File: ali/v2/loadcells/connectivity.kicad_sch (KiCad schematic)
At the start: 27 parts, among them J7 Conn_01x03, J8 Vertical Ethernet, U3 TJA1462ATK, U4 LAN8742AI, Y3 25 MHz

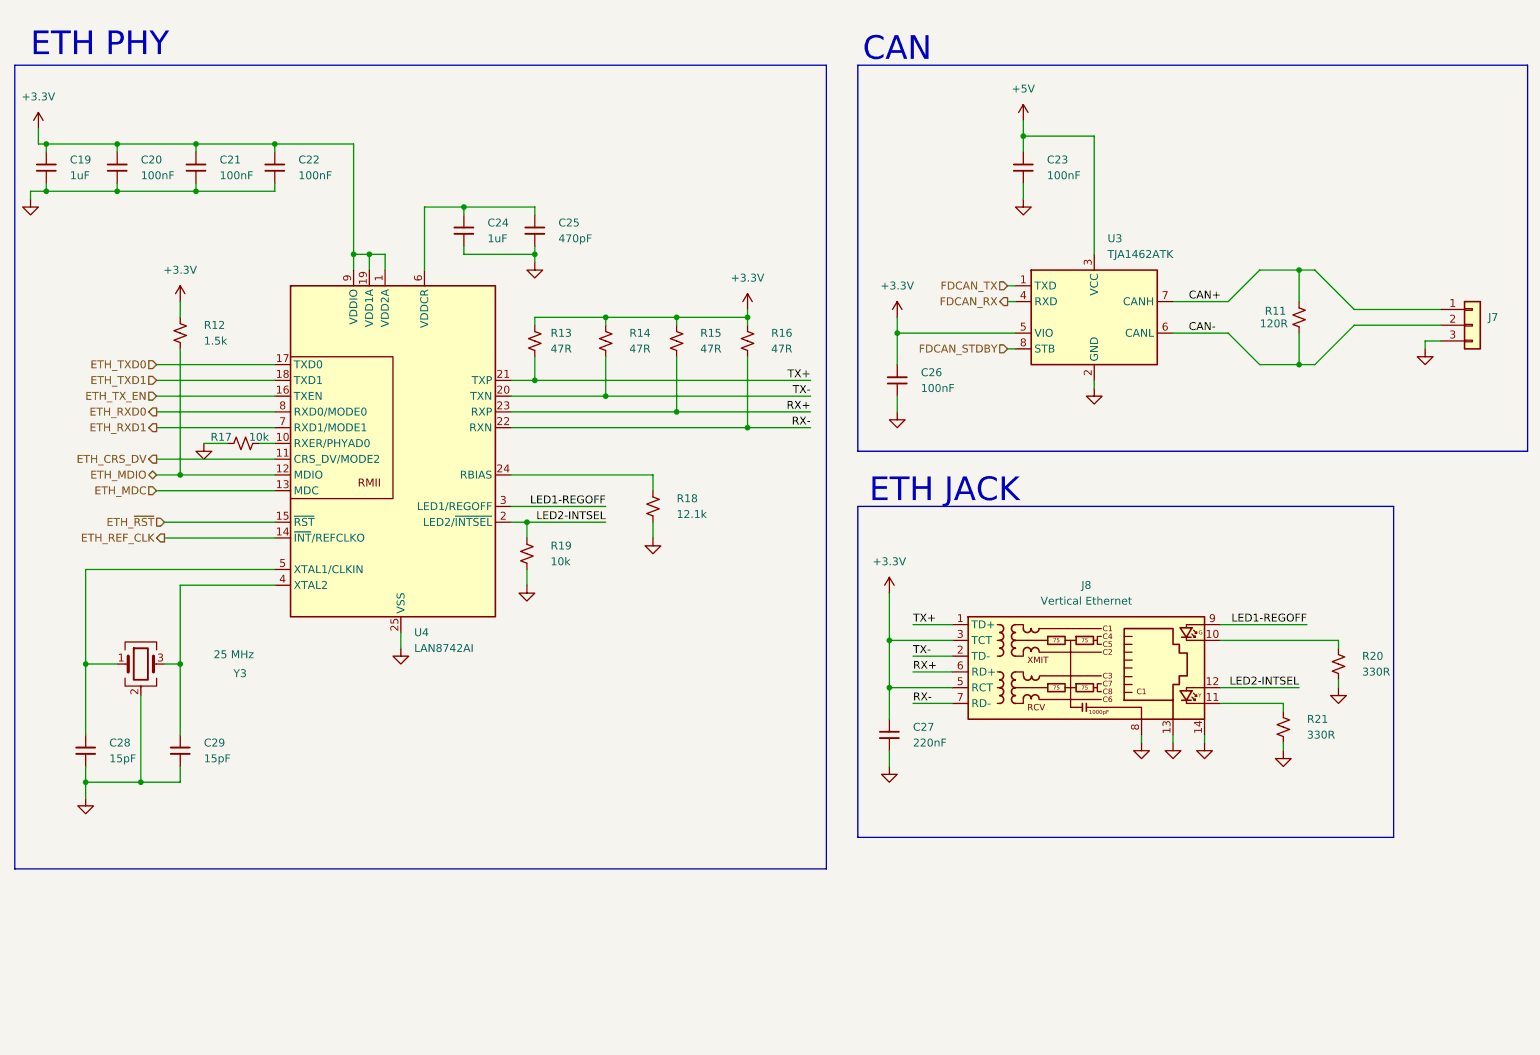
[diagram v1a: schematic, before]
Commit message: Begin prep for second board review
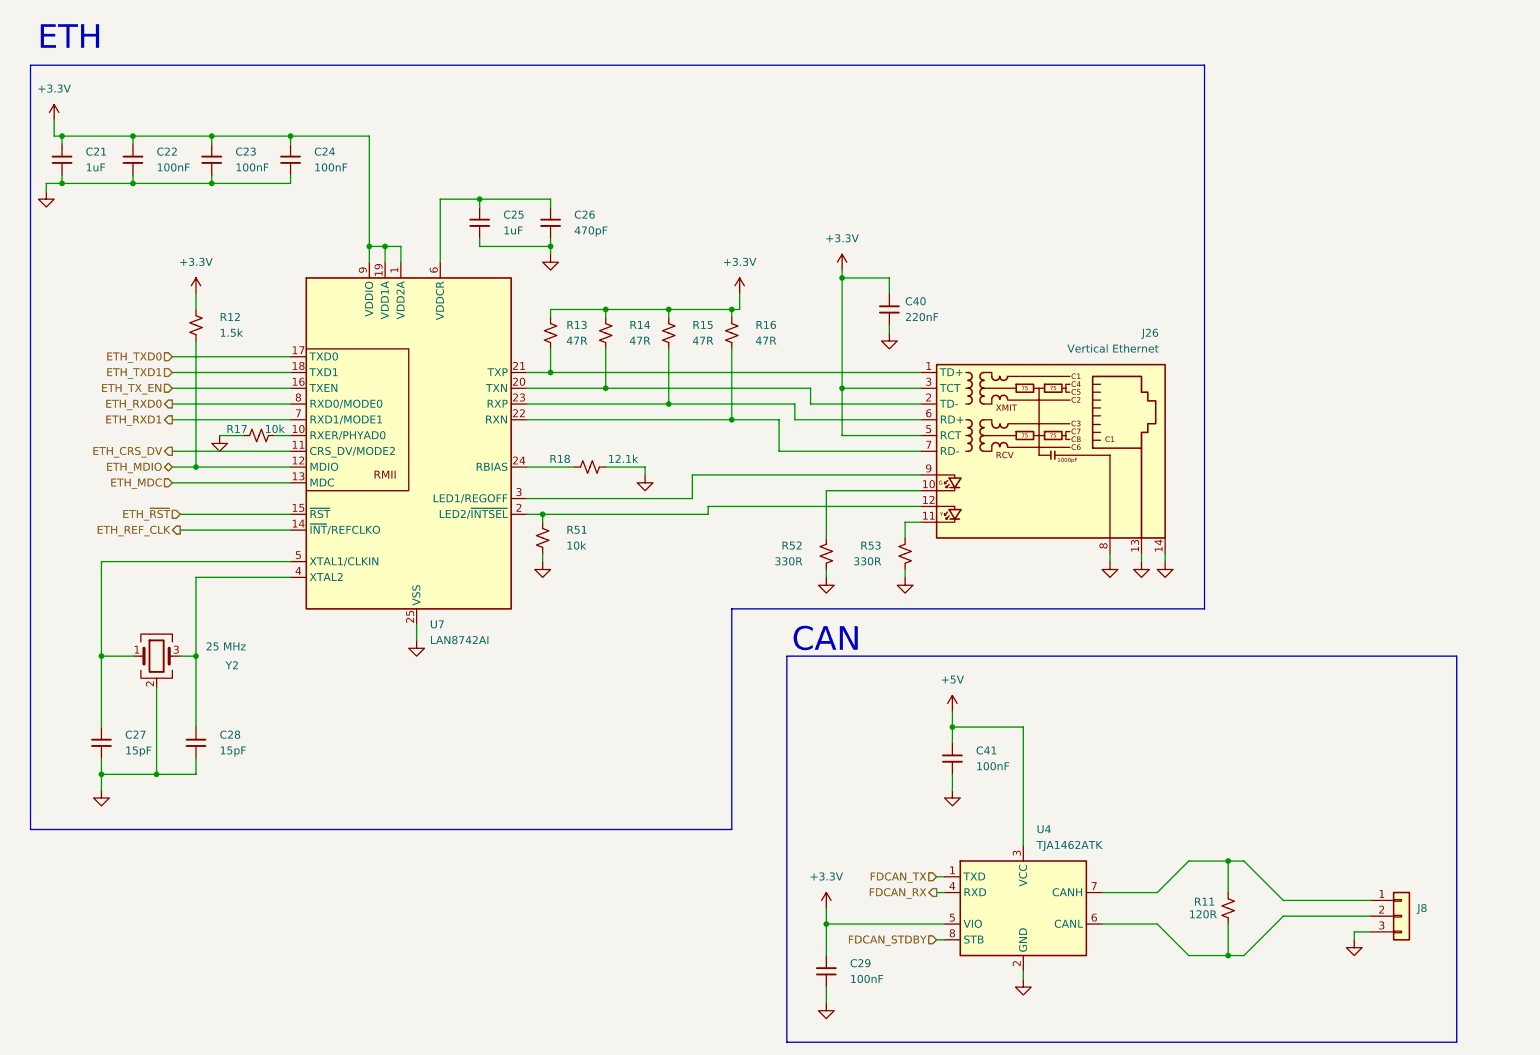
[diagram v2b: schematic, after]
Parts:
- removed C19: 1uF, APRL_Passive:C_0603, symbol Device:C_Small
- removed C20: 100nF, APRL_Passive:C_0603, symbol Device:C_Small
- removed J7: Conn_01x03, APRL_Connector_Molex:Molex_CLIK-Mate_503159-0301_1x03-1MP_P1.50mm_Vertical, symbol Connector_Generic:Conn_01x03
- removed J8: Vertical Ethernet, APRL_Connector:RJ45_Hanrun_HY951180A_Vertical, symbol APRL_Connector:RJ45_Hanrun_HY951180A
- removed R19: 10k, APRL_Passive:R_0603, symbol Device:R_Small_US
- removed R20, R21: 330R, APRL_Passive:R_0603, symbol Device:R_Small_US
- removed U3: TJA1462ATK, APRL_Package_QFN:HVSON-8-1EP_3x3mm_P0.65mm_EP1.6x2.4mm_ThermalVias, symbol APRL_Comms:TJA1462ATK
- removed U4: LAN8742AI, APRL_Package_QFN:VQFN-24-1EP_4x4mm_P0.5mm_EP2.5x2.5mm_ThermalVias, symbol APRL_Comms:LAN8742A
- removed Y3: 25 MHz, APRL_Passive:3225-4P-L, symbol Device:Crystal_GND24
- added C40: 220nF, APRL_Passive:C_0603, symbol Device:C_Small
- added C41: 100nF, APRL_Passive:C_0603, symbol Device:C_Small
- added J26: Vertical Ethernet, APRL_Connector:RJ45_Hanrun_HY951180A_Vertical, symbol APRL_Connector:RJ45_Hanrun_HY951180A
- added J8: Conn_01x03, APRL_Connector_Molex:Molex_CLIK-Mate_503159-0301_1x03-1MP_P1.50mm_Vertical, symbol Connector_Generic:Conn_01x03
- added R51: 10k, APRL_Passive:R_0603, symbol Device:R_Small_US
- added R52, R53: 330R, APRL_Passive:R_0603, symbol Device:R_Small_US
- added U4: TJA1462ATK, APRL_Package_QFN:HVSON-8-1EP_3x3mm_P0.65mm_EP1.6x2.4mm_ThermalVias, symbol APRL_Comms:TJA1462ATK
- added U7: LAN8742AI, APRL_Package_QFN:VQFN-24-1EP_4x4mm_P0.5mm_EP2.5x2.5mm_ThermalVias, symbol APRL_Comms:LAN8742A
- added Y2: 25 MHz, APRL_Passive:3225-4P-L, symbol Device:Crystal_GND24
- C21: value 100nF -> 1uF; MPN GRM188R72A104KA35 -> GRM188D72A105KE01
- C24: value 1uF -> 100nF; MPN GRM188D72A105KE01 -> GRM188R72A104KA35
- C25: value 470pF -> 1uF; MPN GRM1885C1H471JA01 -> GRM188D72A105KE01
- C26: value 100nF -> 470pF; MPN GRM188R72A104KA35 -> GRM1885C1H471JA01
- C27: value 220nF -> 15pF; MPN GRM188R71H224KAC4 -> GRM1885C2E150FW07
- C29: value 15pF -> 100nF; MPN GRM1885C2E150FW07 -> GRM188R72A104KA35
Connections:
- net +3.3V: now also C23.1, C24.1, C29.1, C40.1, J26.3 (TCT), J26.5 (RCT), U4.5 (VIO), U7.1 (VDD2A), U7.19 (VDD1A), U7.9 (VDDIO); no longer C26.1, C27.1
- net +5V: now also C41.1, U4.3 (VCC); no longer C23.1
- net ETH_CRS_DV: now also U7.11 (CRS_DV/MODE2)
- net ETH_MDC: now also U7.13 (MDC)
- net ETH_MDIO: now also U7.12 (MDIO)
- net ETH_REF_CLK: now also U7.14 (~{INT}/REFCLKO)
- net ETH_RXD0: now also U7.8 (RXD0/MODE0)
- net ETH_RXD1: now also U7.7 (RXD1/MODE1)
- net ETH_TXD0: now also U7.17 (TXD0)
- net ETH_TXD1: now also U7.18 (TXD1)
- net ETH_TX_EN: now also U7.16 (TXEN)
- net ETH_~{RST}: now also U7.15 (~{RST})
- net FDCAN_RX: now also U4.4 (RXD)
- net FDCAN_STDBY: now also U4.8 (STB)
- net FDCAN_TX: now also U4.1 (TXD)
- net GND: now also C40.2, C41.2, J26.13, J26.14, J26.8, J8.3 (Pin_3), R51.2, R52.2, R53.2, U4.2 (GND), U4.9 (GND), U7.25 (VSS), Y2.2 (G), Y2.4 (G)
- net at C28.1: now also U7.4 (XTAL2), Y2.3
- net at C25.1: now also C26.1, U7.6 (VDDCR); no longer C24.1
- net at R17.2: now also U7.10 (RXER/PHYAD0)
- net at R18.1: now also U7.24 (RBIAS)
- net CAN+: no longer names the net of R11.2
- net CAN+: now also J8.1 (Pin_1), U4.7 (CANH)
- net CAN-: no longer names the net of R11.1
- net CAN-: now also J8.2 (Pin_2), U4.6 (CANL)
- net RX+: no longer names the net of R15.2
- net RX+: now also J26.6 (RD+), U7.23 (RXP)
- net RX-: no longer names the net of R16.2
- net RX-: now also J26.7 (RD-), U7.22 (RXN)
- net TX+: no longer names the net of R13.2
- net TX+: now also J26.1 (TD+), U7.21 (TXP)
- net TX-: no longer names the net of R14.2
- net TX-: now also J26.2 (TD-), U7.20 (TXN)
- new net: C27.1, U7.5 (XTAL1/CLKIN), Y2.1
- new net: J26.10, R52.1
- new net: J26.12, R51.1, U7.2 (LED2/~{INTSEL})
- new net: J26.9, U7.3 (LED1/REGOFF)
- new net: J26.11, R53.1
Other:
- note added: "ETH"
- note removed: "ETH JACK"
- note removed: "ETH PHY"
